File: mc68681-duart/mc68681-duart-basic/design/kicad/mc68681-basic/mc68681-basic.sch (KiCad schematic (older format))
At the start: 30 parts, among them IC1 XR68C681CJTR-F, IC2 74HCT245, IC3 74HCT245, IC4 74HCT245, IC5 74125, IC6 IC6_DECO.PLD, IC7 IC7_UART_.PLD, J1 Conn_02x32_Odd_Even, J2 EXTBUS, J3 UART_A, J4 UART_B, Q1 Crystal

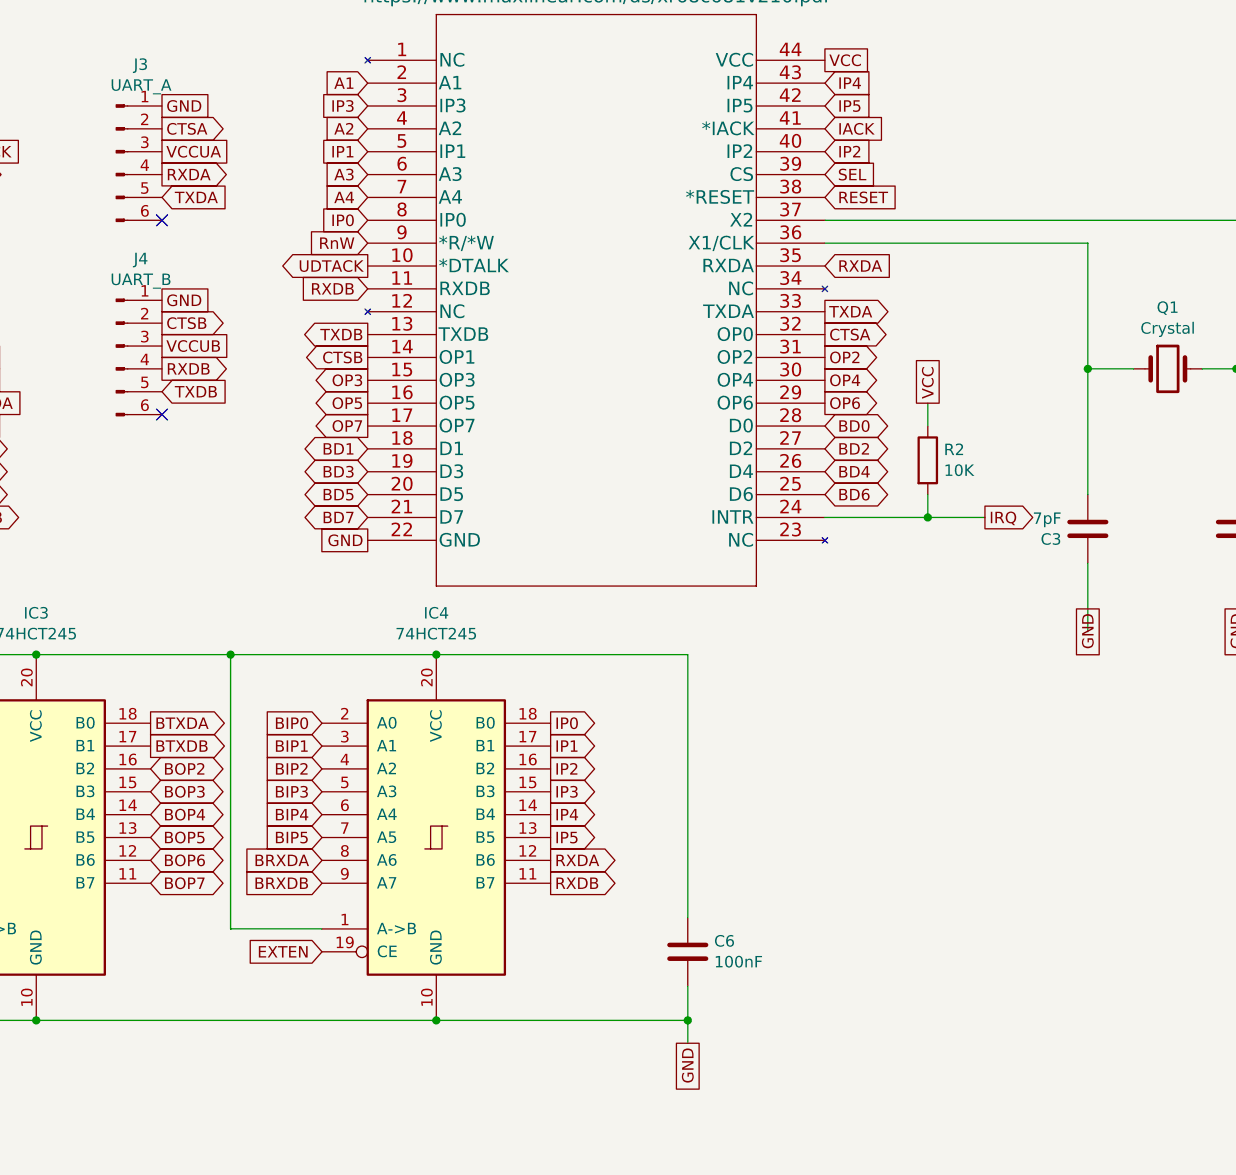
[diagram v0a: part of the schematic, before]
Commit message: DUART 2.1
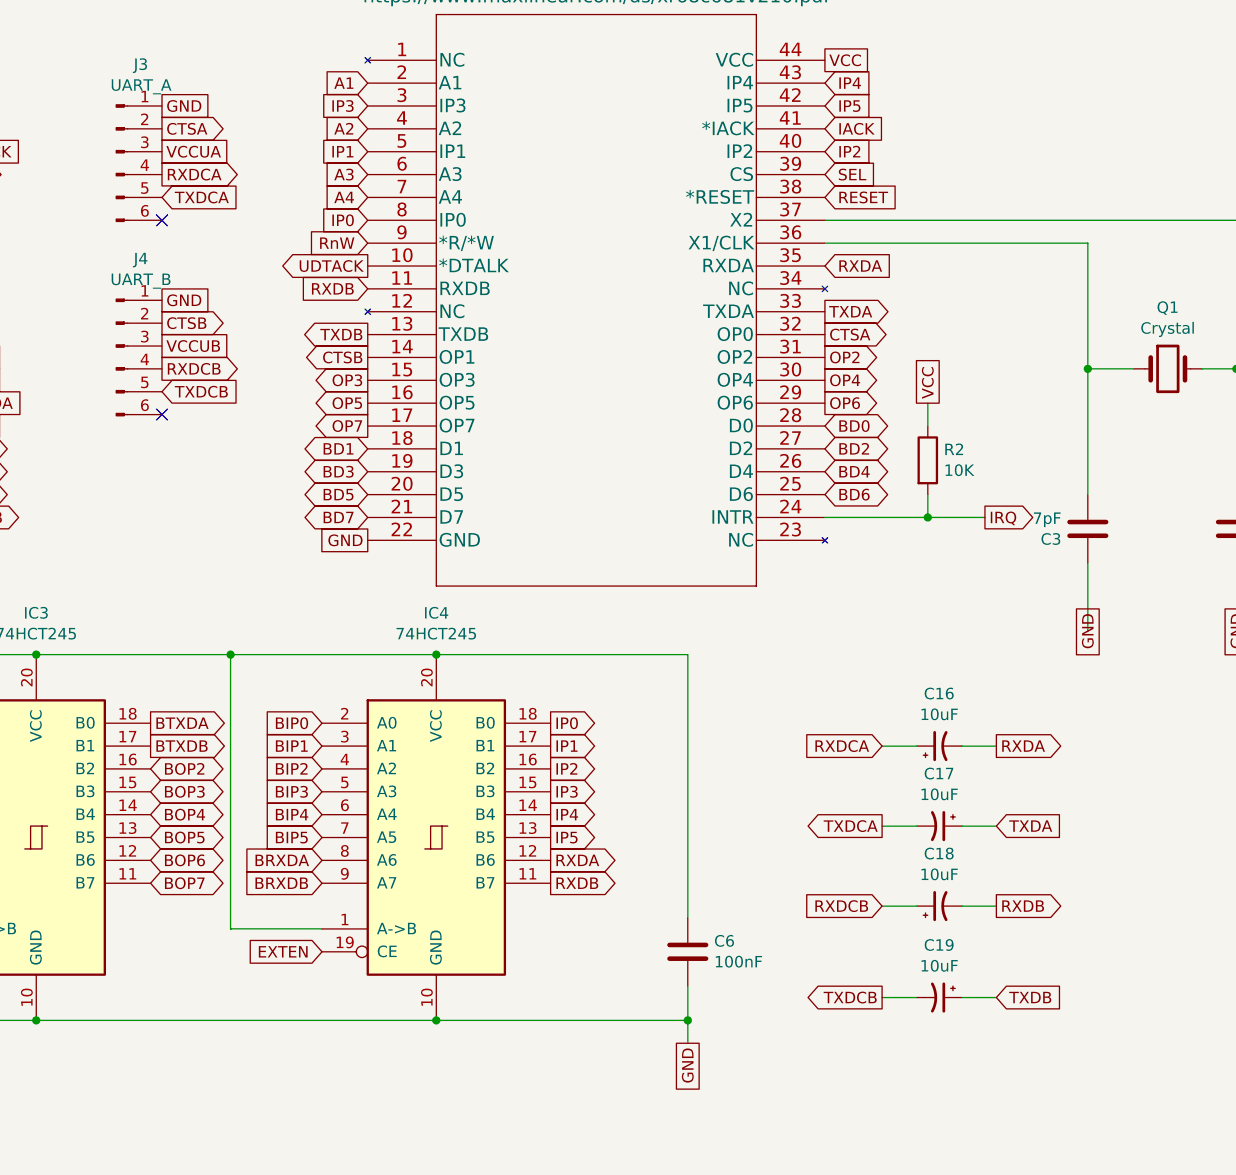
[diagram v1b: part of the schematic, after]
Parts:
- added C16, C17, C18, C19: 10uF, Capacitor_THT:CP_Radial_D5.0mm_P2.00mm, symbol Device:CP1_Small
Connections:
- net RXDA: now also C16.2; no longer J3.4 (Pin_4)
- net RXDB: now also C18.2; no longer J4.4 (Pin_4)
- net TXDA: now also C17.1; no longer J3.5 (Pin_5)
- net TXDB: now also C19.1; no longer J4.5 (Pin_5)
- new net RXDCA: C16.1, J3.4 (Pin_4)
- new net RXDCB: C18.1, J4.4 (Pin_4)
- new net TXDCA: C17.2, J3.5 (Pin_5)
- new net TXDCB: C19.2, J4.5 (Pin_5)
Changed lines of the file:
@@
 Sheet 1 1
 Title "ROSCO_M68K MC68681 DUART EXPANSION"
-Date "2021-03-01"
-Rev "2"
+Date "2021-06-26"
+Rev "2.1"
 Comp "The Really Old School Company Limited"
 Comment1 ""
@@
 CTSA
 Text GLabel 2500 3700 2    50   Input ~ 0
-TXDA
+TXDCA
 Text GLabel 2500 3600 2    50   Output ~ 0
-RXDA
+RXDCA
 NoConn ~ 2500 3800
 Text GLabel 10550 5350 2    50   UnSpc ~ 0
@@
 CTSB
 Text GLabel 2500 4550 2    50   Input ~ 0
-TXDB
+TXDCB
 Text GLabel 2500 4450 2    50   Output ~ 0
-RXDB
+RXDCB
 NoConn ~ 2500 4650
 $Comp
@@
 Wire Wire Line
 	8750 5250 9550 5250
+Text GLabel 5650 6100 0    50   Input ~ 0
+RXDCA
+$Comp
+L Device:CP1_Small C16
+U 1 1 60D6C450
+P 5900 6100
+F 0 "C16" V 6128 6100 50  0000 C CNN
+F 1 "10uF" V 6037 6100 50  0000 C CNN
+F 2 "Capacitor_THT:CP_Radial_D5.0mm_P2.00mm" H 5900 6100 50  0001 C CNN
+F 3 "~" H 5900 6100 50  0001 C CNN
+	1    5900 6100
+	0    -1   -1   0
+$EndComp
+$Comp
+L Device:CP1_Small C17
+U 1 1 60D6DFF3
+P 5900 6450
+F 0 "C17" V 5672 6450 50  0000 C CNN
+F 1 "10uF" V 5763 6450 50  0000 C CNN
+F 2 "Capacitor_THT:CP_Radial_D5.0mm_P2.00mm" H 5900 6450 50  0001 C CNN
+F 3 "~" H 5900 6450 50  0001 C CNN
+	1    5900 6450
+	0    1    1    0
+$EndComp
+$Comp
+L Device:CP1_Small C18
+U 1 1 60D73E6D
+P 5900 6800
+F 0 "C18" V 6128 6800 50  0000 C CNN
+F 1 "10uF" V 6037 6800 50  0000 C CNN
+F 2 "Capacitor_THT:CP_Radial_D5.0mm_P2.00mm" H 5900 6800 50  0001 C CNN
+F 3 "~" H 5900 6800 50  0001 C CNN
+	1    5900 6800
+	0    -1   -1   0
+$EndComp
+$Comp
+L Device:CP1_Small C19
+U 1 1 60D797B1
+P 5900 7200
+F 0 "C19" V 5672 7200 50  0000 C CNN
+F 1 "10uF" V 5763 7200 50  0000 C CNN
+F 2 "Capacitor_THT:CP_Radial_D5.0mm_P2.00mm" H 5900 7200 50  0001 C CNN
+F 3 "~" H 5900 7200 50  0001 C CNN
+	1    5900 7200
+	0    1    1    0
+$EndComp
+Text GLabel 5650 6800 0    50   Input ~ 0
+RXDCB
+Text GLabel 6150 6450 2    50   Input ~ 0
+TXDA
+Text GLabel 6150 7200 2    50   Input ~ 0
+TXDB
+Text GLabel 6150 6100 2    50   Output ~ 0
+RXDA
+Text GLabel 6150 6800 2    50   Output ~ 0
+RXDB
+Text GLabel 5650 6450 0    50   Output ~ 0
+TXDCA
+Text GLabel 5650 7200 0    50   Output ~ 0
+TXDCB
+Wire Wire Line
+	5650 6100 5800 6100
+Wire Wire Line
+	6000 6100 6150 6100
+Wire Wire Line
+	5650 6450 5800 6450
+Wire Wire Line
+	6000 6450 6150 6450
+Wire Wire Line
+	5650 6800 5800 6800
+Wire Wire Line
+	6000 6800 6150 6800
+Wire Wire Line
+	5650 7200 5800 7200
+Wire Wire Line
+	6000 7200 6150 7200
 $EndSCHEMATC
